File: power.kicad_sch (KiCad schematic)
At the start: 12 parts, among them U1 AP7363-33D-13

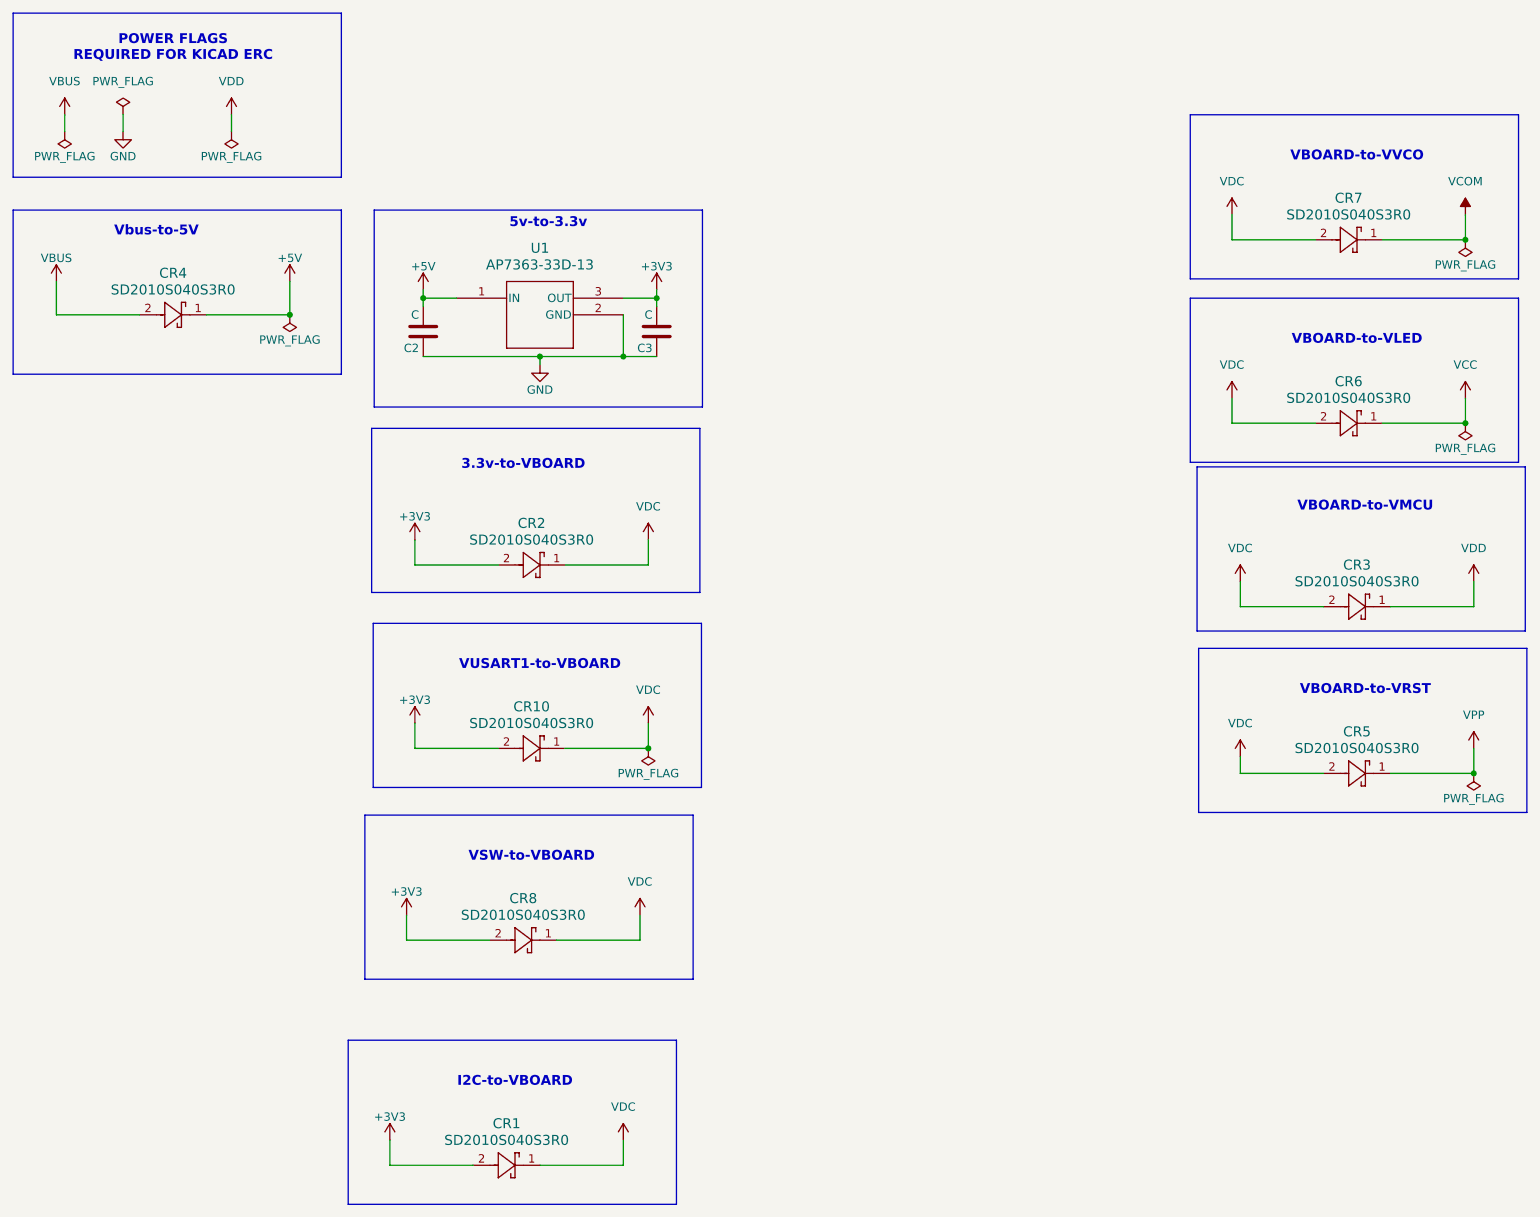
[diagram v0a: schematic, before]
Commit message: added sheets
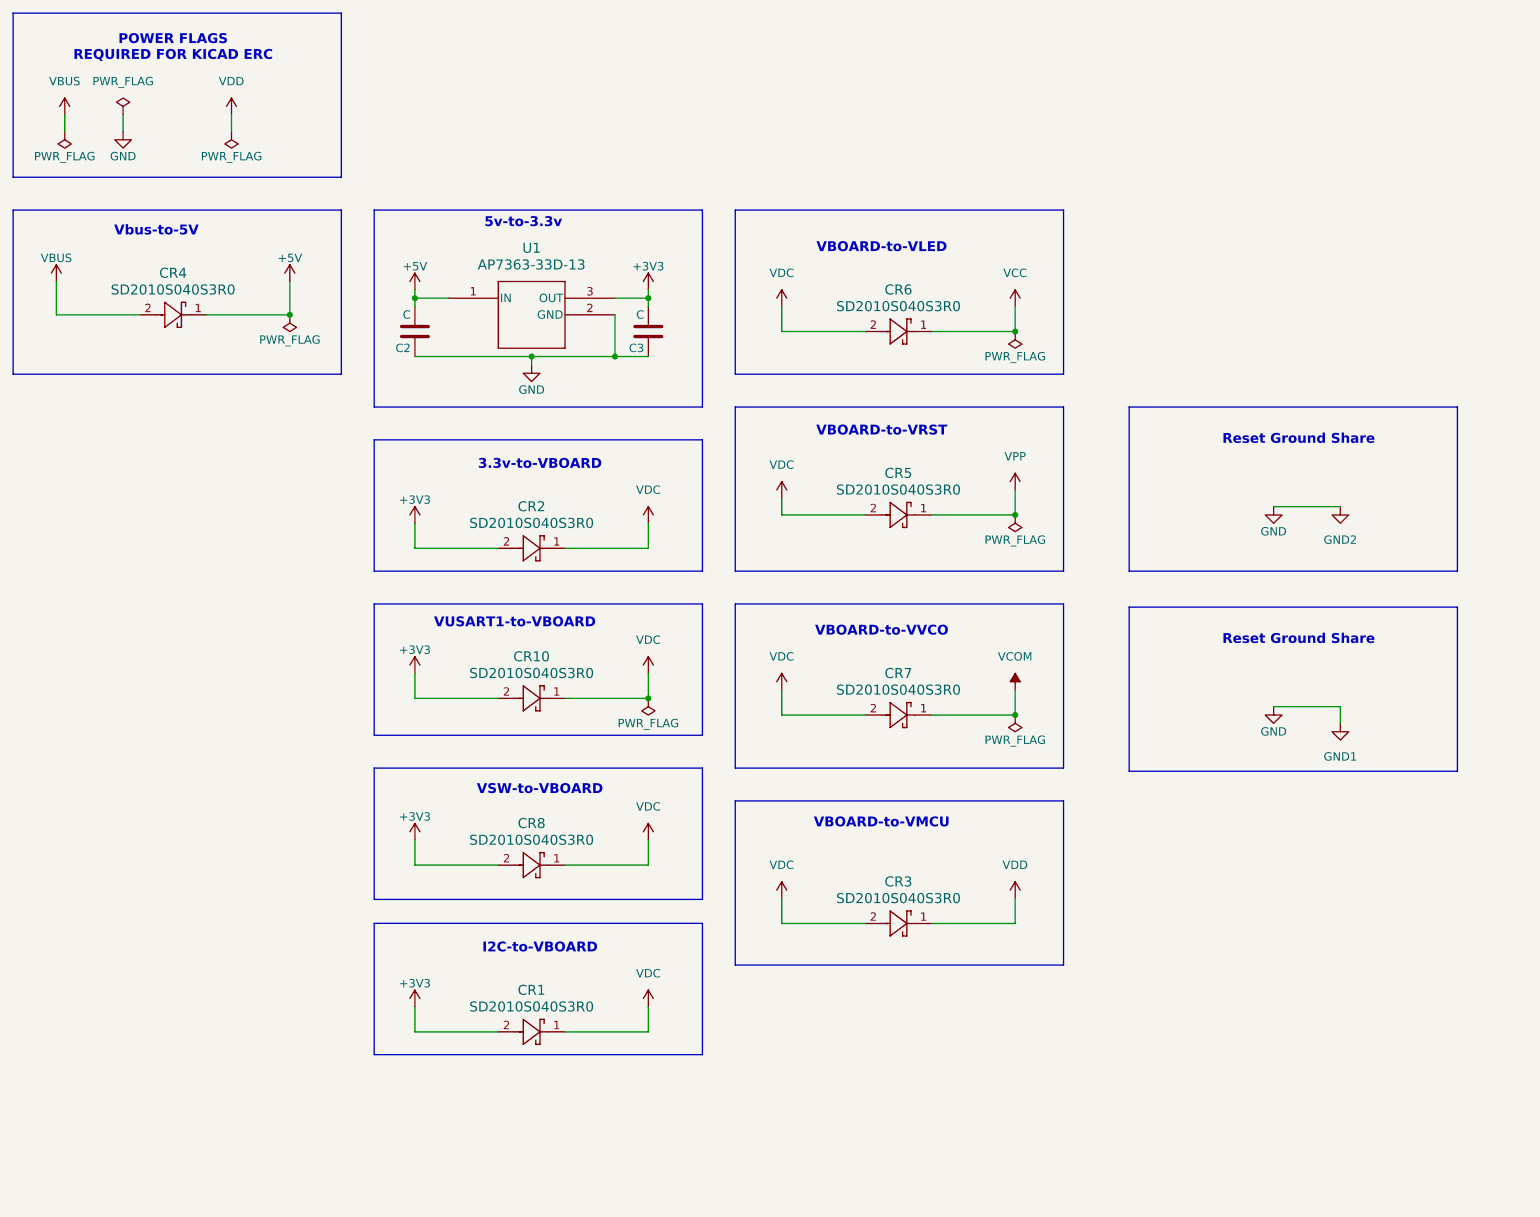
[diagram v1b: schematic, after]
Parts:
- CR1, CR10, CR2, CR3, CR4, CR5, CR6, CR7, CR8: footprint SDO_KAVX_KAV -> DIODE_SCHOTTKY_40V_3A:SDO_KAVX_KAV
- U1: footprint TO252-3L_DIO -> PMIC_VREG_LDO_3.3V:TO252-3L_DIO
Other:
- note added: "Reset Ground Share"
- moved on the sheet: C2, C3, CR1, CR10, CR2, CR3, CR5, CR6, CR7, CR8, U1
